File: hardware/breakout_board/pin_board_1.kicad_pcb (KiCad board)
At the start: 2 copper layers, 49.4 x 94.2 mm, 51 parts, among them P1 CONN_1, P10 CONN_1, P11 CONN_1, P12 CONN_1, P13 CONN_1, P14 CONN_1, P15 CONN_1, P16 CONN_1, P17 CONN_1, P18 CONN_1, P19 CONN_1, P2 CONN_1, P20 CONN_1, P21 CONN_1, P22 CONN_1, P23 CONN_1, P24 CONN_1, P25 CONN_1, P26 CONN_1, P27 CONN_1, P28 CONN_1, P29 CONN_1, P3 CONN_1, P30 CONN_1, P31 CONN_1, P4 CONN_1, P5 CONN_1, P6 CONN_1, P7 CONN_1, P8 CONN_1, P9 CONN_1

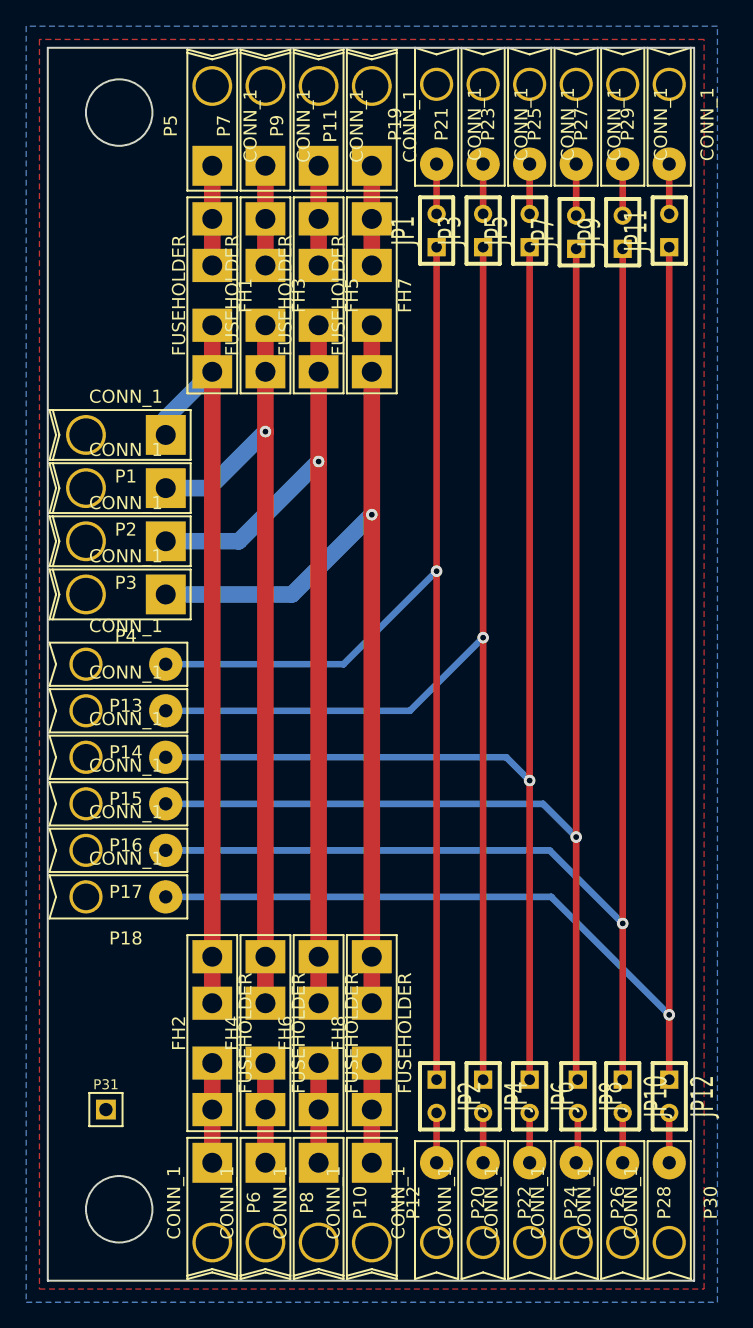
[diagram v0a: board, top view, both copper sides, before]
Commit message: 2nd version
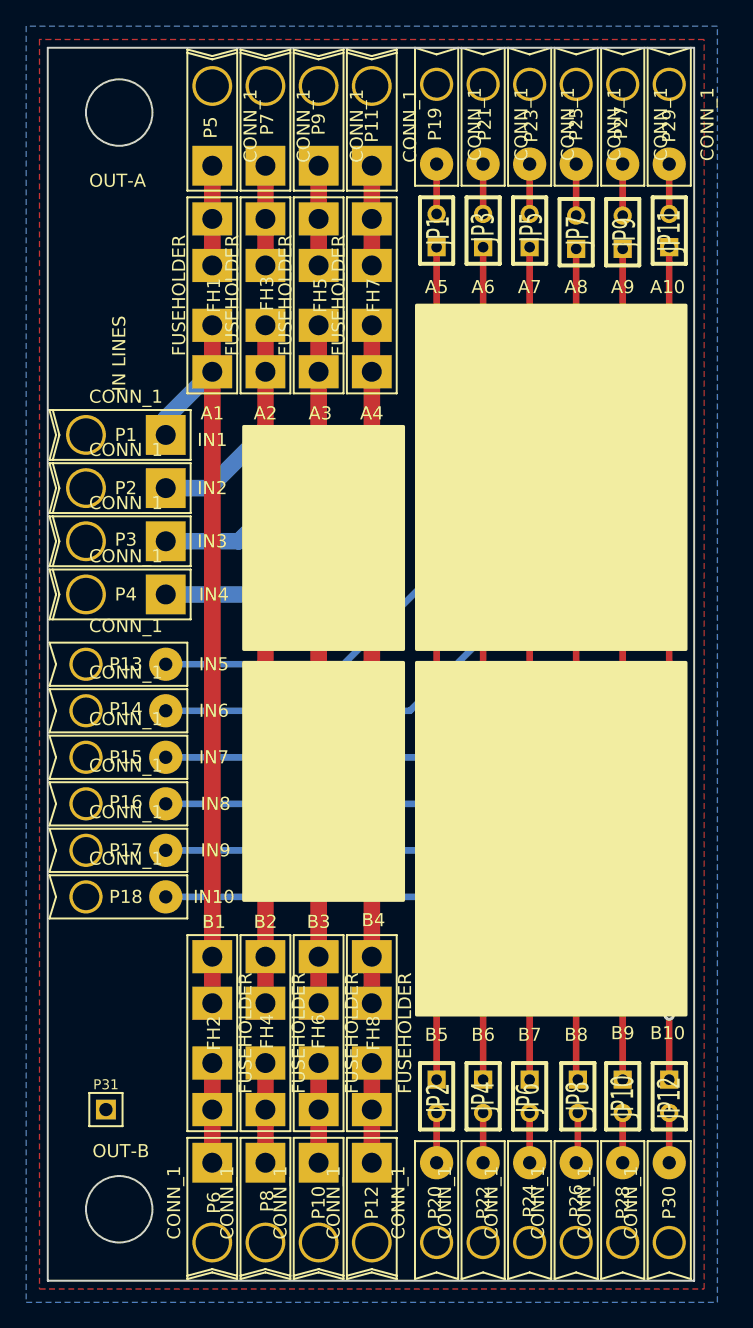
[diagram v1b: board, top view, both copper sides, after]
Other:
- board text added: "A1"
- board text added: "A10"
- board text added: "A2"
- board text added: "A3"
- board text added: "A4"
- board text added: "A5"
- board text added: "A6"
- board text added: "A7"
- board text added: "A8"
- board text added: "A9"
- board text added: "B1"
- board text added: "B10"
- board text added: "B2"
- board text added: "B3"
- board text added: "B4"
- board text added: "B5"
- board text added: "B6"
- board text added: "B7"
- board text added: "B8"
- board text added: "B9"
- board text added: "IN LINES"
- board text added: "IN1"
- board text added: "IN10"
- board text added: "IN2"
- board text added: "IN3"
- board text added: "IN4"
- board text added: "IN5"
- board text added: "IN6"
- board text added: "IN7"
- board text added: "IN8"
- board text added: "IN9"
- board text added: "OUT-A"
- board text added: "OUT-B"
